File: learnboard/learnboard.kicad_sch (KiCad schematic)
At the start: 59 parts, among them SW1 SW_Push, SW10 SW_Push, SW11 SW_Push, SW12 SW_Push, SW13 SW_Push, SW14 SW_Push, SW15 SW_Push, SW16 SW_Push, SW17 RotaryEncoder_Switch_MP, SW2 SW_Push, SW3 SW_Push, SW4 SW_Push, SW5 SW_Push, SW6 SW_Push, SW7 SW_Push, SW8 SW_Push, SW9 SW_Push, U1 PCM5100

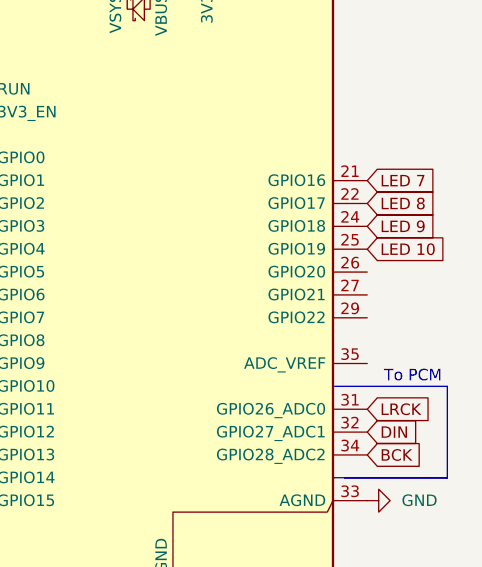
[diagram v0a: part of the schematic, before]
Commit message: Worked on firmware and webapp
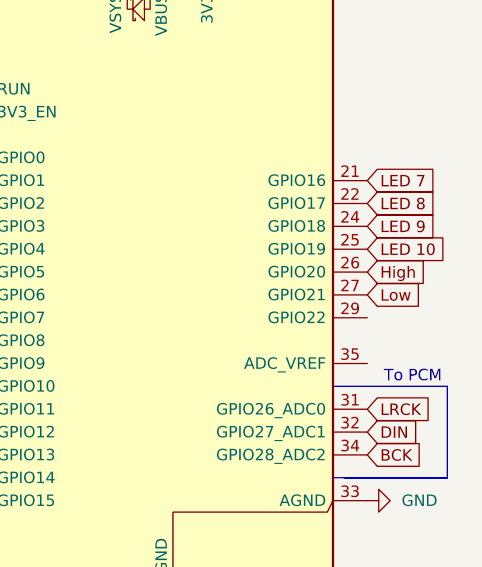
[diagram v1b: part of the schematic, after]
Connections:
- net High: now also A1.26 (GPIO20)
- net Low: now also A1.27 (GPIO21)
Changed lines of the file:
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@@
+		)
+	)
+	(global_label "Low"
+		(shape input)
+		(at 264.16 101.6 0)
+		(fields_autoplaced yes)
+		(effects
+			(font
+				(size 1.27 1.27)
+			)
+			(justify left)
+		)
+		(property "Intersheetrefs" "${INTERSHEET_REFS}"
+			(at 270.6528 101.6 0)
+			(effects
+				(font
+					(size 1.27 1.27)
+				)
+				(justify left)
+				(hide yes)
+			)
 		)
 	)
@@
 			(effects
 				(font
+					(size 1.27 1.27)
+				)
+				(justify left)
+				(hide yes)
+			)
+		)
+	)
+	(global_label "High"
+		(shape input)
+		(at 264.16 99.06 0)
+		(fields_autoplaced yes)
+		(effects
+			(font
+				(size 1.27 1.27)
+			)
+			(justify left)
+		)
+		(property "Intersheetrefs" "${INTERSHEET_REFS}"
+			(at 271.3785 99.06 0)
+			(effects
+				(font
